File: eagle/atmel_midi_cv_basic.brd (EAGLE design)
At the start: 100 x 80 mm, 46 parts, among them IC1 TL074P, Q2 2N3904, U1 ATMEGA328P_PDIP

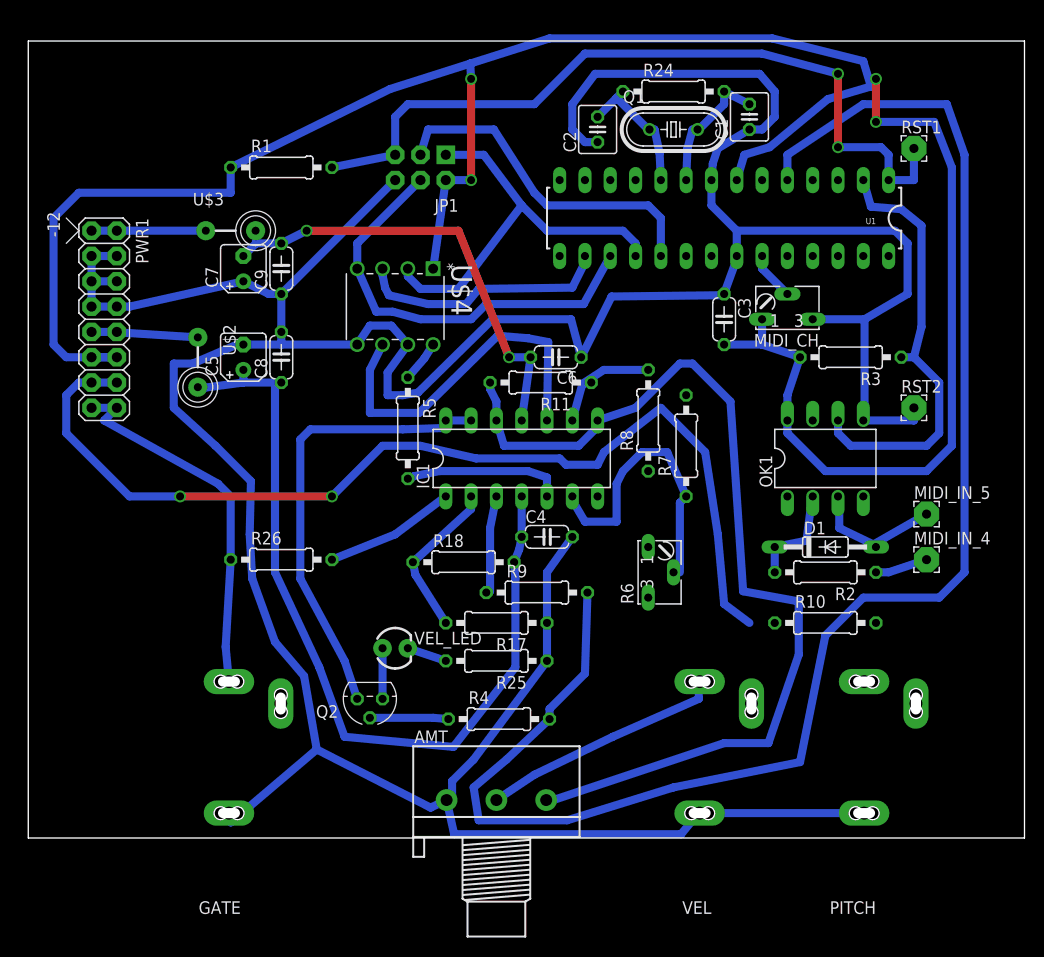
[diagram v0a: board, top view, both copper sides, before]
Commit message: sloppy routed
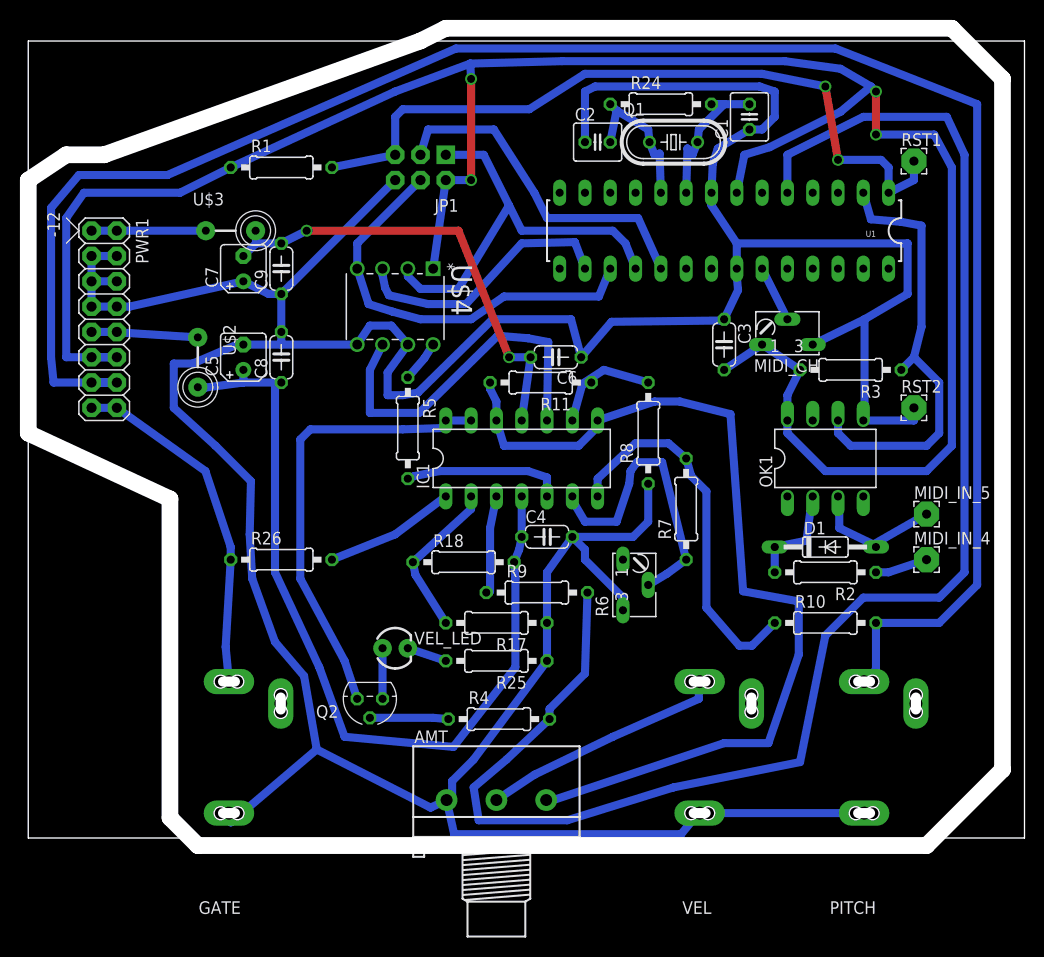
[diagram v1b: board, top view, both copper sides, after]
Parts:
- moved R7 6.35 mm to (66.0, 33.0)
- moved R6 2.84 mm to (59.7, 25.4)
- moved C3 2.54 mm to (69.8, 49.5)
- moved MIDI_CH 2.54 mm to (76.2, 49.5)
- moved R24 1.80 mm to (63.5, 73.7)
- moved C2 1.27 mm to (57.1, 69.8), turned to 0 degrees
- moved Q1 1.27 mm to (64.8, 69.8)
- moved RST1 1.27 mm to (88.9, 67.9)
- moved R3 1.27 mm to (82.5, 47.0)
- moved R8 1.27 mm to (62.2, 40.6)
- moved U1 1.27 mm to (69.8, 61.0)
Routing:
- net N$9: track 101.4 -> 191.0 mm, vias 2 -> 0
- net N$27: track 0.00 -> 37.9 mm
- net GND: track 376.5 -> 395.6 mm
- net +5V: track 234.4 -> 226.2 mm
- net N$17: track 97.1 -> 92.7 mm
- net N$43: track 78.6 -> 75.1 mm
- net N$4: track 13.5 -> 16.6 mm
- net N$31: track 37.8 -> 35.0 mm
- net N$25: track 25.5 -> 27.1 mm
- net N$5: track 13.9 -> 14.9 mm
- net N$26: track 43.3 -> 42.3 mm
- net N$45: track 41.3 -> 42.2 mm
- net N$19: track 4.86 -> 5.68 mm
- net N$22: track 157.7 -> 157.2 mm
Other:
- board size 100 x 80 mm -> 100 x 82 mm

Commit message: almost
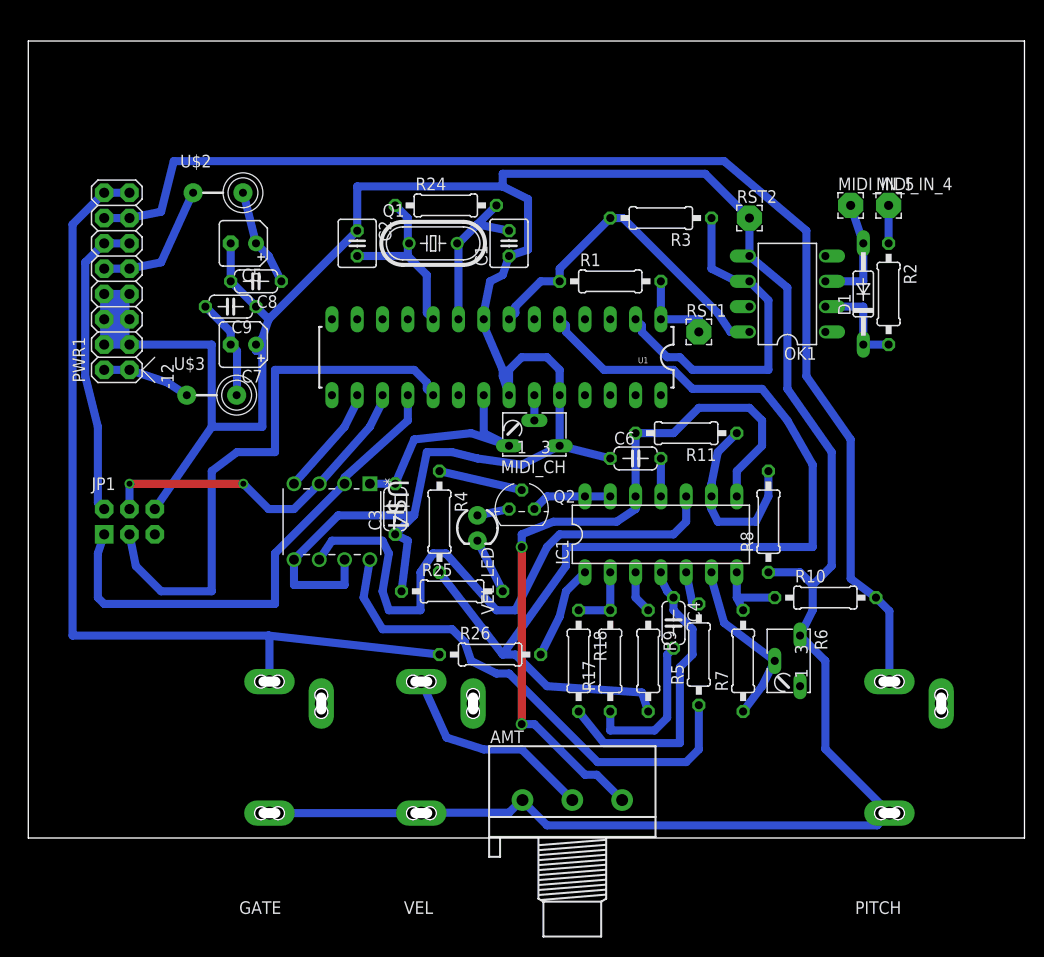
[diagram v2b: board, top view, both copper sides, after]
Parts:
- moved JP1 46.0 mm to (10.2, 31.8), turned to 0 degrees
- moved R5 37.0 mm to (67.3, 18.4), turned to 90 degrees
- moved C3 36.9 mm to (36.8, 33.0), turned to 90 degrees
- moved MIDI_IN_4 35.8 mm to (86.4, 63.5)
- moved R1 34.9 mm to (58.4, 55.9)
- moved MIDI_IN_5 31.9 mm to (82.5, 63.5)
- moved R2 28.7 mm to (86.4, 54.6), turned to 270 degrees
- moved VEL 27.9 mm to (44.5, 0.00)
- moved RST1 27.6 mm to (67.3, 50.8)
- moved MIDI_CH 27.4 mm to (50.8, 39.4)
- moved C1 27.3 mm to (48.3, 59.7)
- moved C2 26.2 mm to (33.0, 59.7), turned to 270 degrees
- moved Q1 26.2 mm to (40.6, 59.7)
- moved U1 26.2 mm to (47.0, 48.3)
- moved D1 25.7 mm to (83.8, 54.6), turned to 90 degrees
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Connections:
- net +5V: now also U1.21
- net GND: now also U1.24
- net N$25: now also U$4.4; no longer U$4.3
- net N$26: now also U$4.3; no longer U$4.4
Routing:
- net +5V: track 226.2 -> 88.6 mm, vias 4 -> 0
- net N$43: track 75.1 -> 8.89 mm, vias 2 -> 0
- net N$9: track 191.0 -> 125.6 mm
- net N$31: track 35.0 -> 89.9 mm
- net N$22: track 157.2 -> 106.3 mm
- net N$2: track 4.18 -> 50.2 mm
- net +12V: track 85.1 -> 40.5 mm
- net N$21: track 45.4 -> 8.15 mm
- net -12V: track 46.0 -> 14.1 mm, vias 2 -> 0
- net N$27: track 37.9 -> 7.77 mm
- net N$14: track 36.2 -> 59.4 mm
- net N$10: track 34.3 -> 56.5 mm
- net N$17: track 92.7 -> 74.9 mm, vias 0 -> 2
- net GND: track 395.6 -> 379.0 mm
- net N$25: track 27.1 -> 11.1 mm
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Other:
- board size 100 x 82 mm -> 100 x 80 mm
